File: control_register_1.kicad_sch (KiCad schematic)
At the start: 8 parts, among them U10 74LS375D, U11 74HC02, U13 74HC21D, U14 74HC21D, U15 74HC21D, U5 74HC08, U7 74HC04D, U9 74LS375D

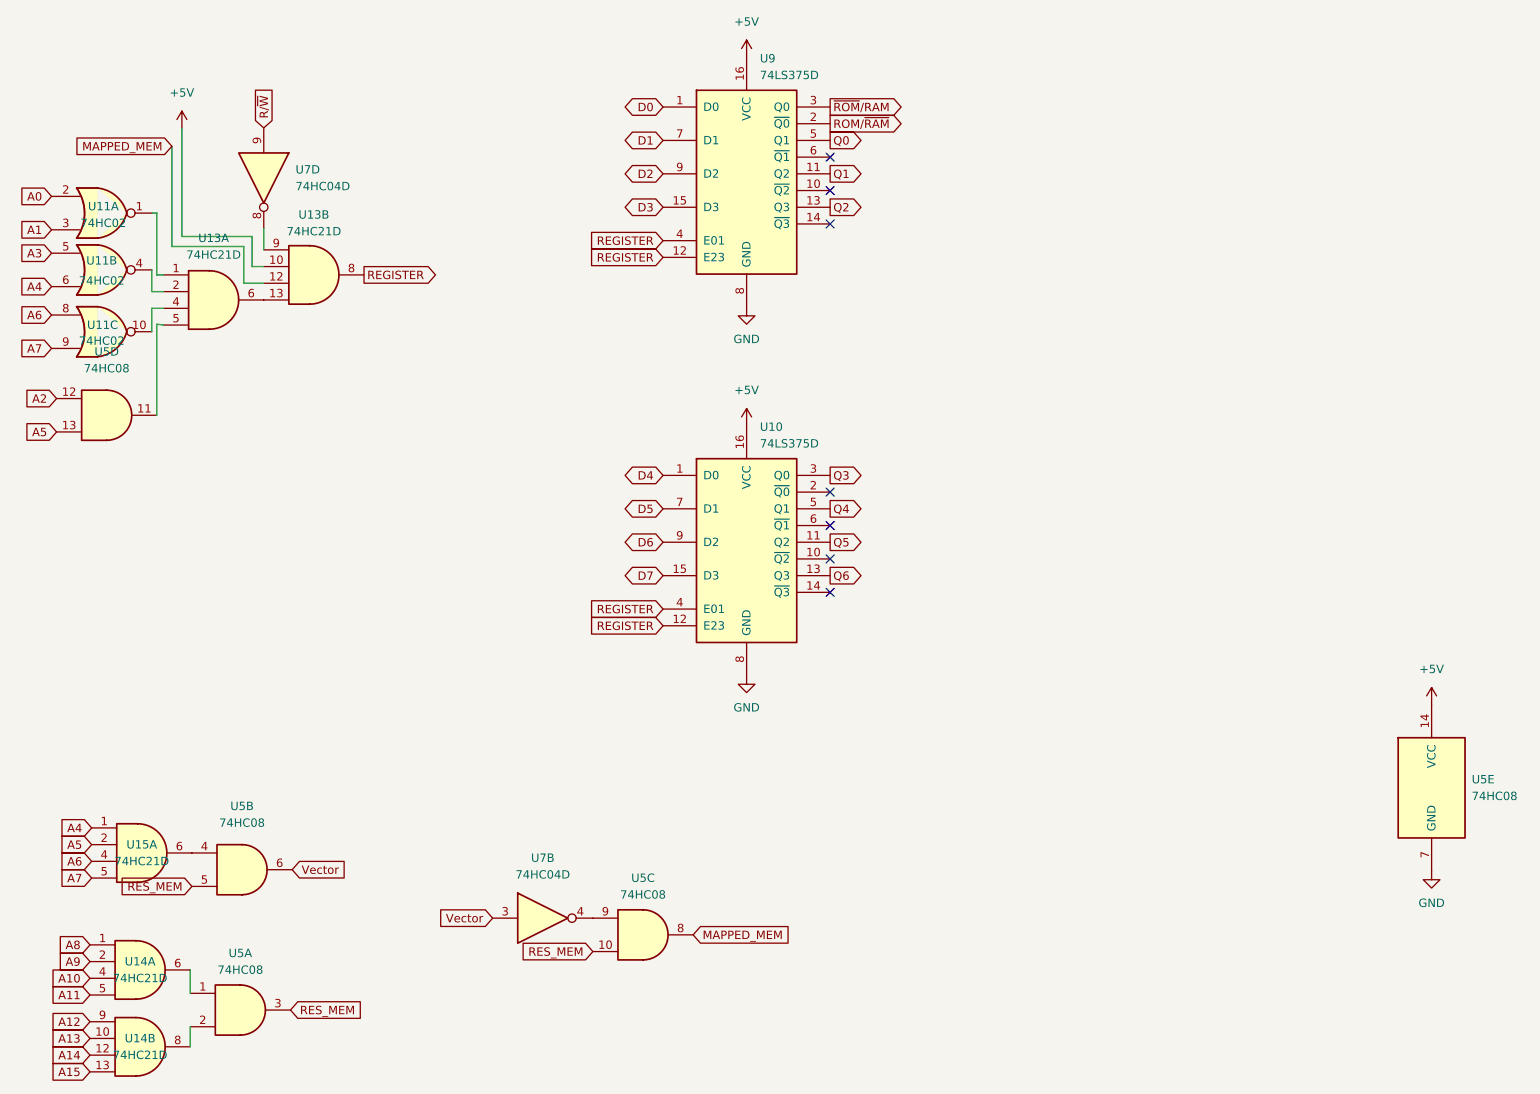
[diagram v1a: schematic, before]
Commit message: convert to discrete clock
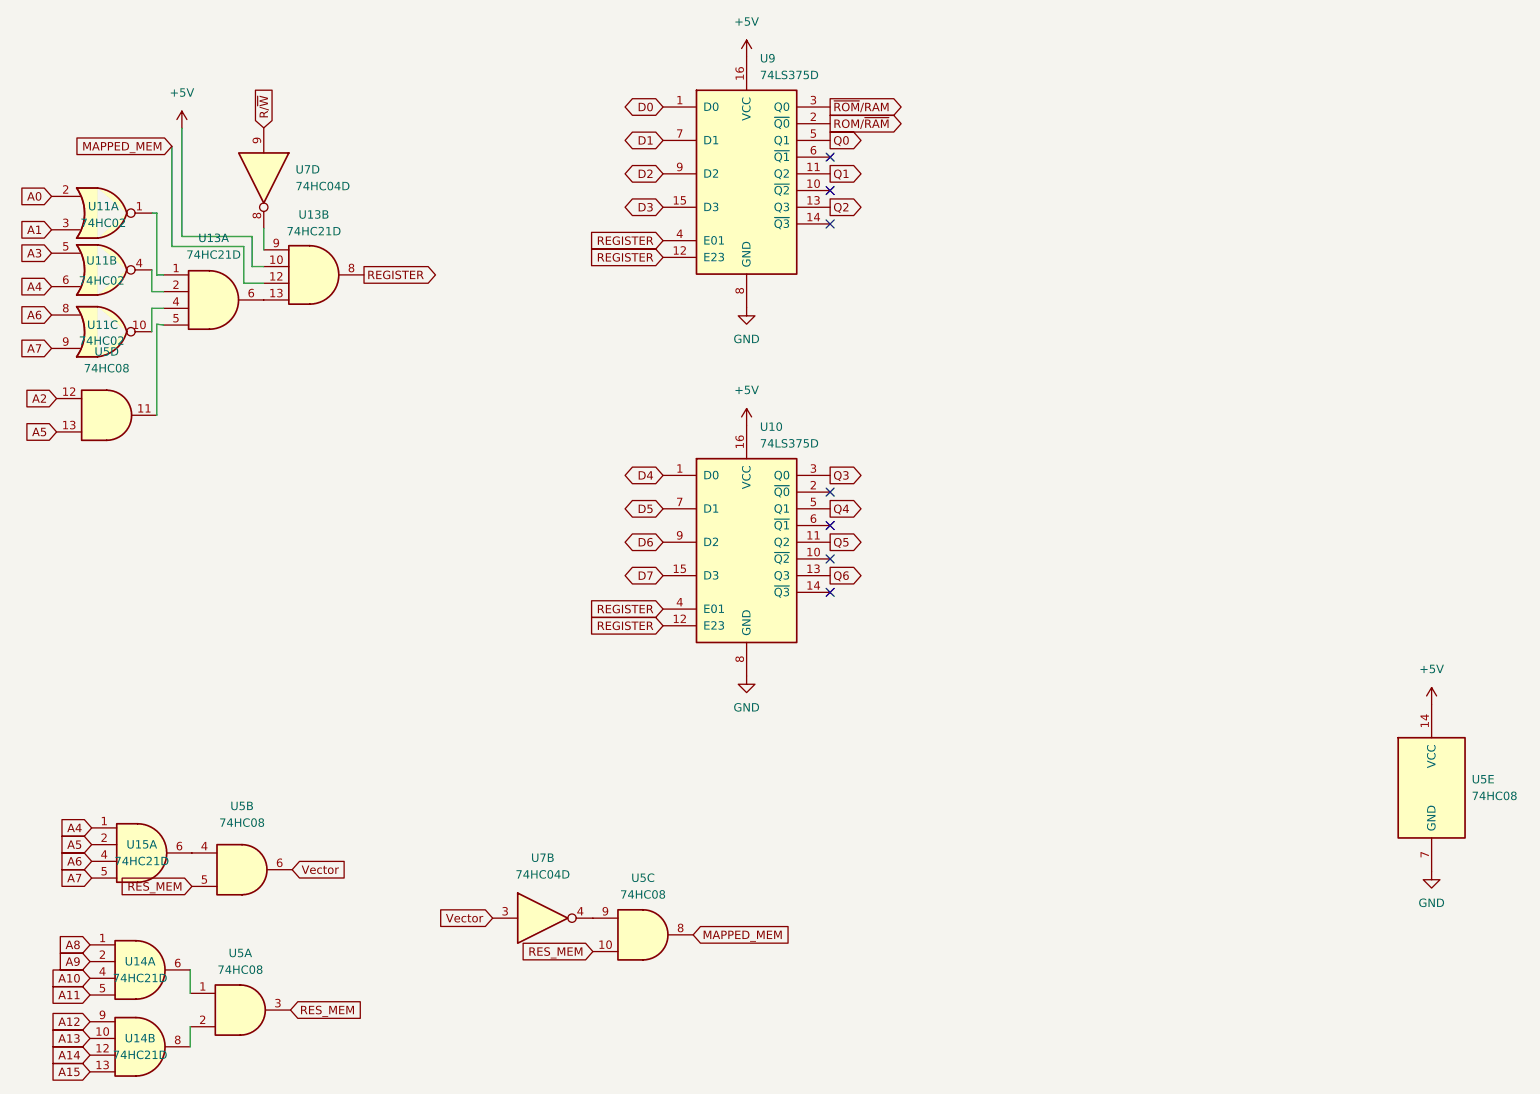
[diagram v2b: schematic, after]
